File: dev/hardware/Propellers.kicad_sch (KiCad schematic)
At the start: 17 parts, among them J201 CPU PGMR, J202 GPU PGMR, J203 SPARE GPU HDR, J204 SPARE CPU HDR, SW201 CPU ~{RES}, SW202 GPU ~{RES}, SW203 DEBUG, U1 P8X32A-D40, Y1 6.5MHz

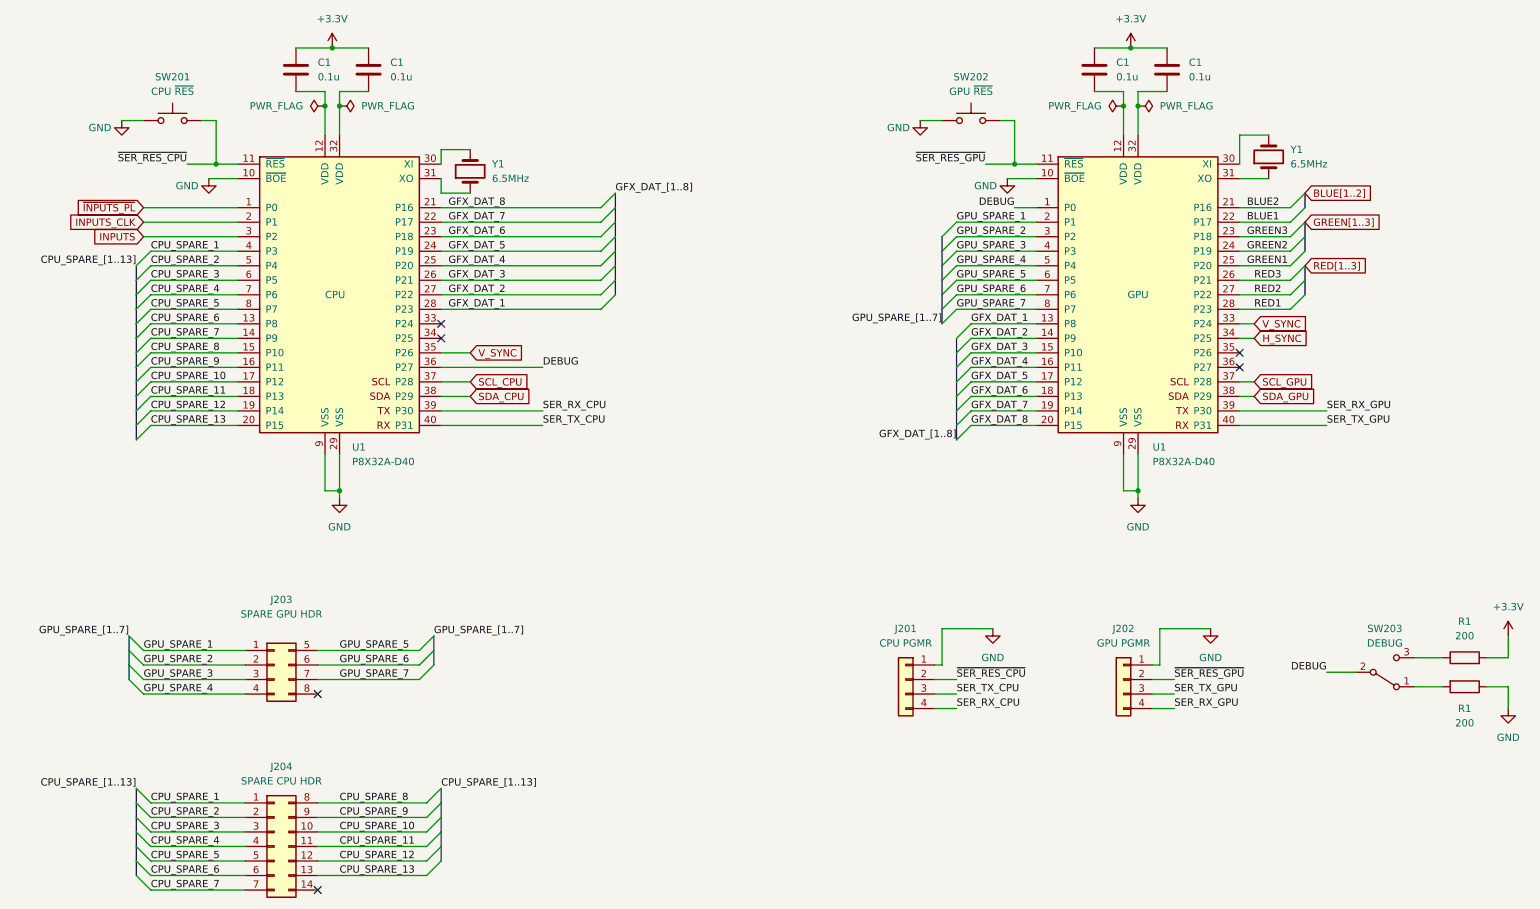
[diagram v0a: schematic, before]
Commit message: Finalized review schematic & pcb
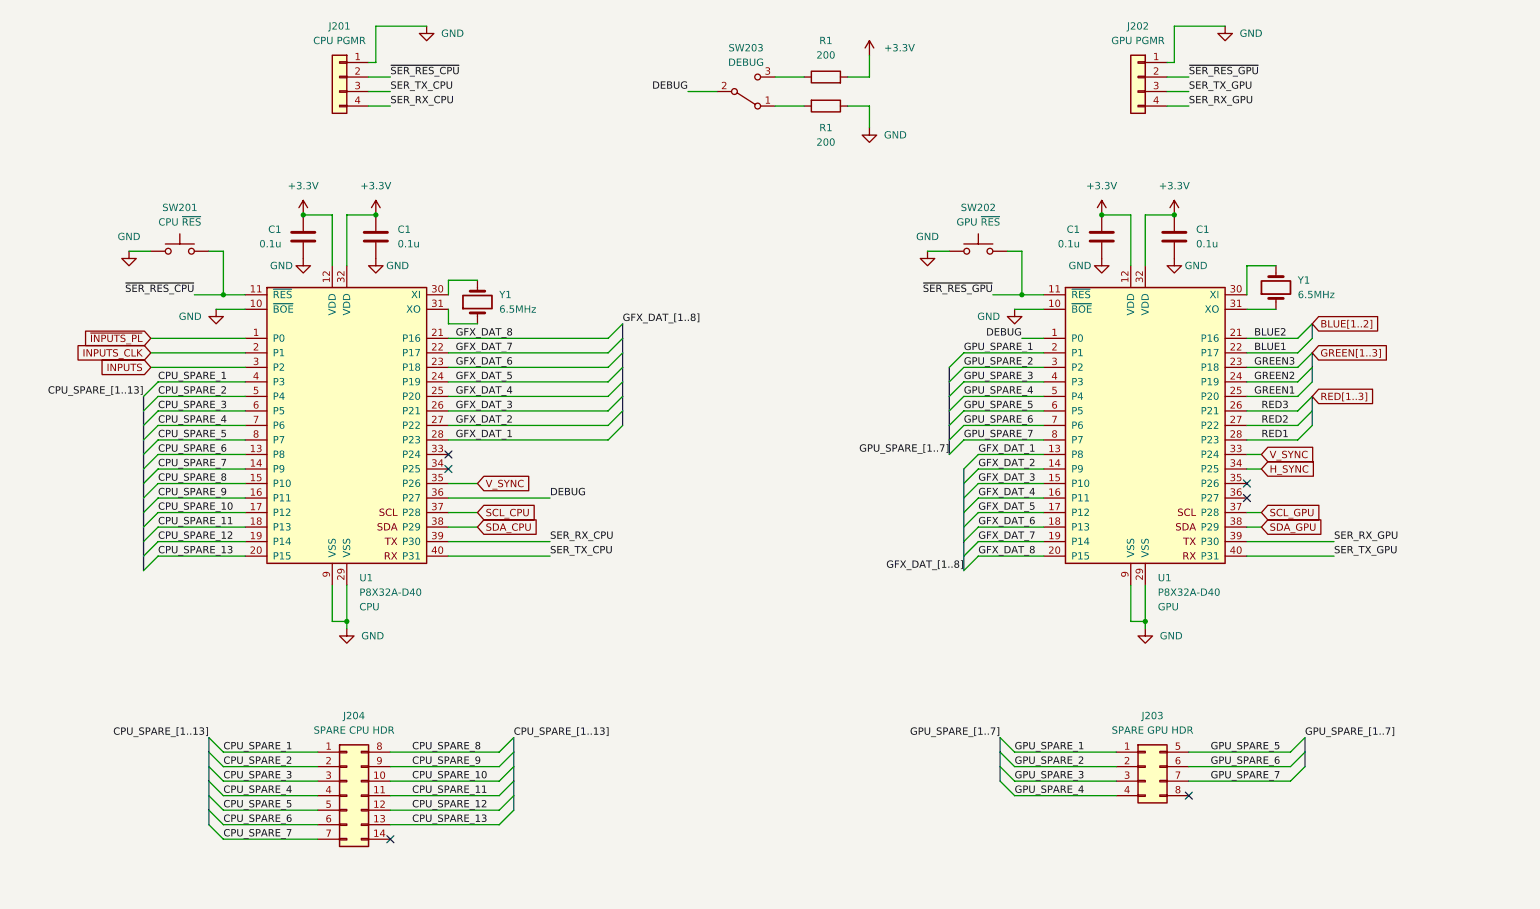
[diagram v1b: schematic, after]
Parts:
- removed C1 (x4): 0.1u, Capacitor_THT:C_Disc_D3.4mm_W2.1mm_P2.50mm, symbol Device:C
- added C1 (x4): 0.1u, Capacitor_THT:C_Disc_D3.4mm_W2.1mm_P2.50mm, symbol Device:C
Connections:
- net +3.3V: now also U1.12 (VDD), U1.12 (VDD), U1.32 (VDD), U1.32 (VDD), C1.2, C1.2, C1.2, C1.2
- net GND: now also C1.1, C1.1, C1.1, C1.1
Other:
- moved on the sheet: J201, J202, J203, J204, R1, SW201, SW202, SW203, U1, Y1
